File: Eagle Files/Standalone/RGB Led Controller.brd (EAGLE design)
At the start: 71.1 x 63.2 mm, 26 parts, among them IC1 7805TV, U1 ATMEGA328P_PDIP, X1 Max 12V in

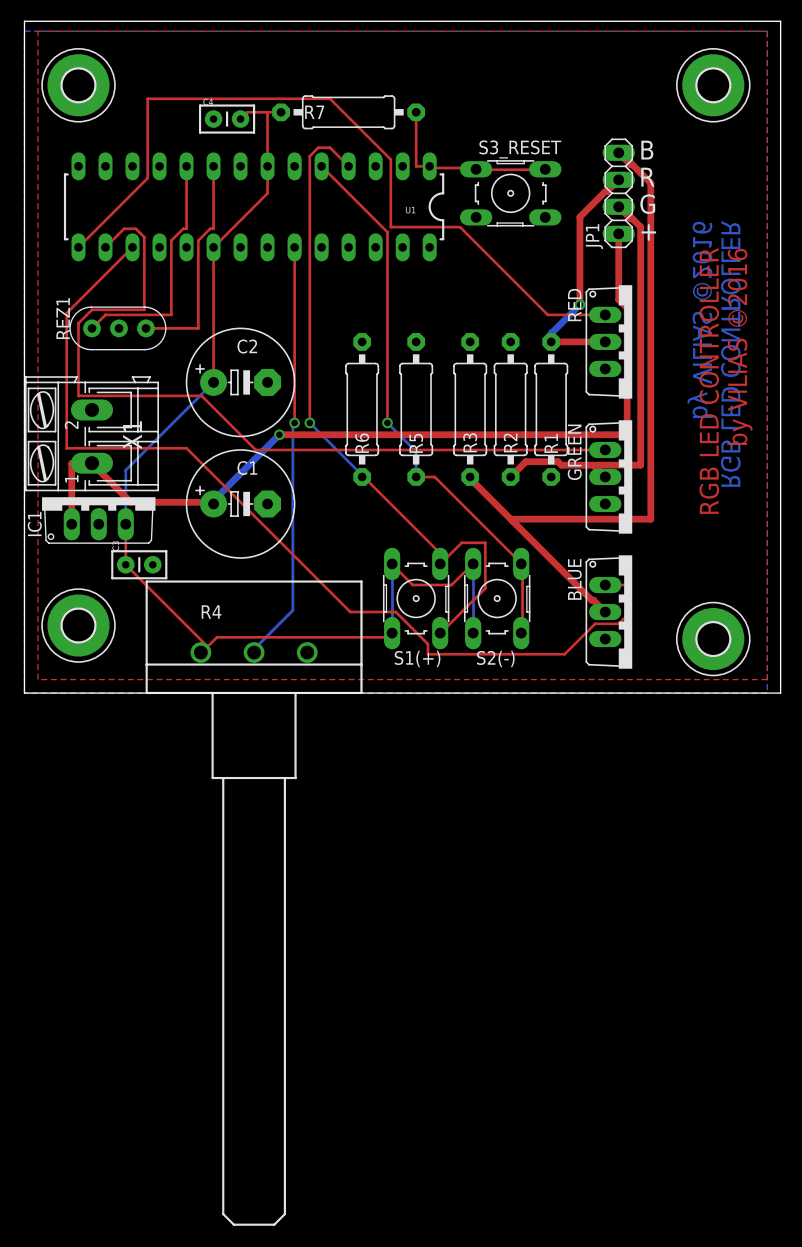
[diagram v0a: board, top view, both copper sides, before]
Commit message: update stand alone
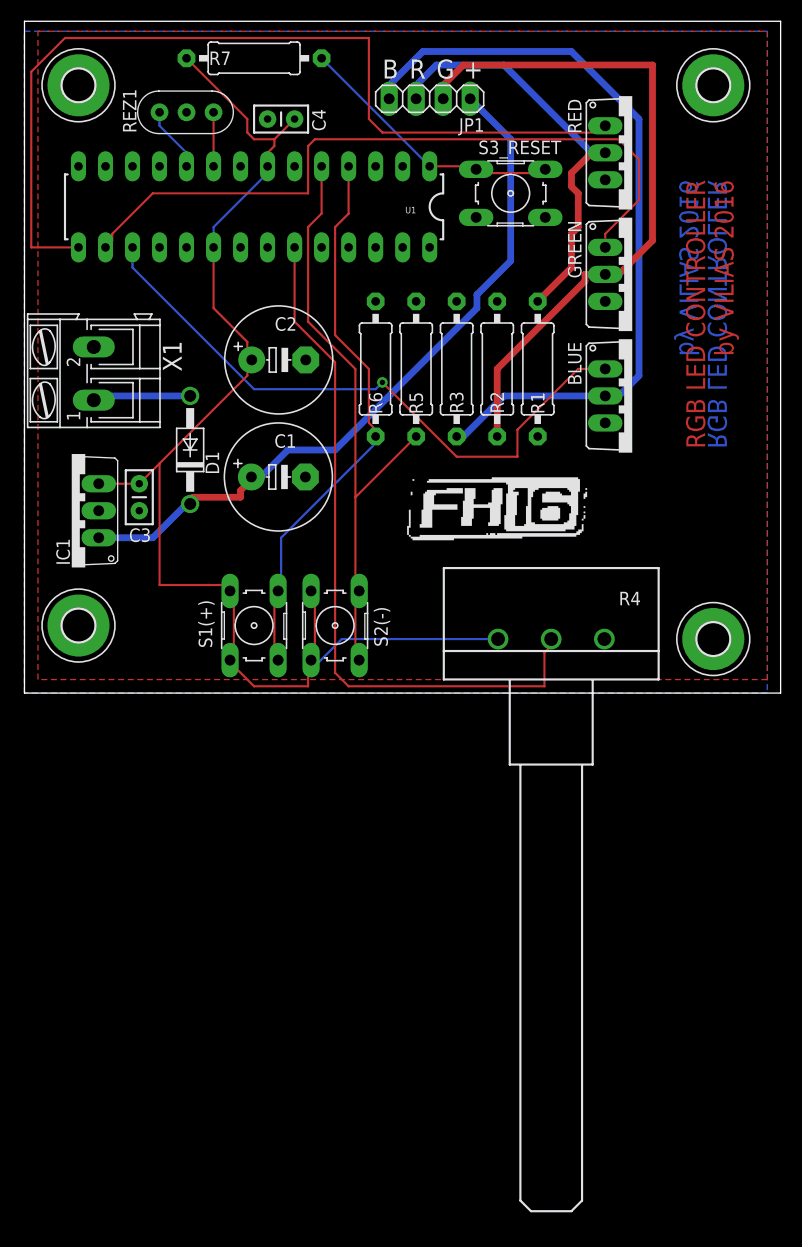
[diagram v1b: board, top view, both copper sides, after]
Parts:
- added D1: 1N4004, diode:DO41-10
- moved R4 28.0 mm to (49.5, 5.08)
- moved REZ1 21.3 mm to (15.2, 54.6)
- moved BLUE 20.3 mm to (54.6, 27.9)
- moved JP1 19.9 mm to (38.1, 55.9), turned to 180 degrees
- moved GREEN 19.0 mm to (54.6, 39.4)
- moved RED 17.8 mm to (54.6, 50.8)
- moved S2(-) 15.5 mm to (29.2, 6.35)
- moved S1(+) 15.5 mm to (21.6, 6.35)
- moved R7 10.2 mm to (21.6, 59.7)
- moved C3 7.73 mm to (10.8, 19.7), turned to 270 degrees
- moved X1 5.93 mm to (6.52, 30.1)
- moved C4 5.08 mm to (25.4, 54.0)
- moved C1 4.37 mm to (23.9, 20.3)
- moved C2 4.17 mm to (23.9, 31.3)
- moved R1 4.02 mm to (48.3, 30.5)
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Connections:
- new net N$11: D1.A, X1.1
- net +12V: now also D1.C; no longer X1.1
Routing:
- net N$5: track 89.0 -> 59.2 mm, vias 0 -> 1
- net N$9: track 39.7 -> 66.5 mm, vias 1 -> 0
- net N$7: track 39.7 -> 64.6 mm
- net N$8: track 23.0 -> 41.1 mm, vias 1 -> 0
- net +5V: track 104.8 -> 121.8 mm
- net N$2: track 22.7 -> 6.13 mm
- net N$1: track 20.9 -> 5.08 mm
- net +12V: track 81.7 -> 68.0 mm, vias 1 -> 0
- net N$3: track 71.8 -> 85.0 mm
- net N$13: track 63.9 -> 52.9 mm, vias 1 -> 0
- net N$11: track 0.00 -> 9.21 mm
- net N$4: track 76.7 -> 67.7 mm
- net N$10: track 17.4 -> 25.9 mm
- net N$6: track 66.9 -> 72.4 mm
- net N$12: track 52.8 -> 57.6 mm, vias 1 -> 0
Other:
- board text added: "RGB LED CONTROLLER by VILIAS 2016"
- board text removed: "RGB LED CONTROLLER by VILIAS ©2016"
